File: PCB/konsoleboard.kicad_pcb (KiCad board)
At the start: 2 copper layers, 73.8 x 116.7 mm, 12 parts, among them SW1 SW_Wuerth_450301014042, SW10 SW_Push, SW2 SW_Push, SW3 SW_Wuerth_450301014042, SW5 SW_Push, SW6 SW_Push, SW7 SW_Push, SW8 SW_Push, SW9 SW_Wuerth_450301014042, U3 CR2013-MI2120

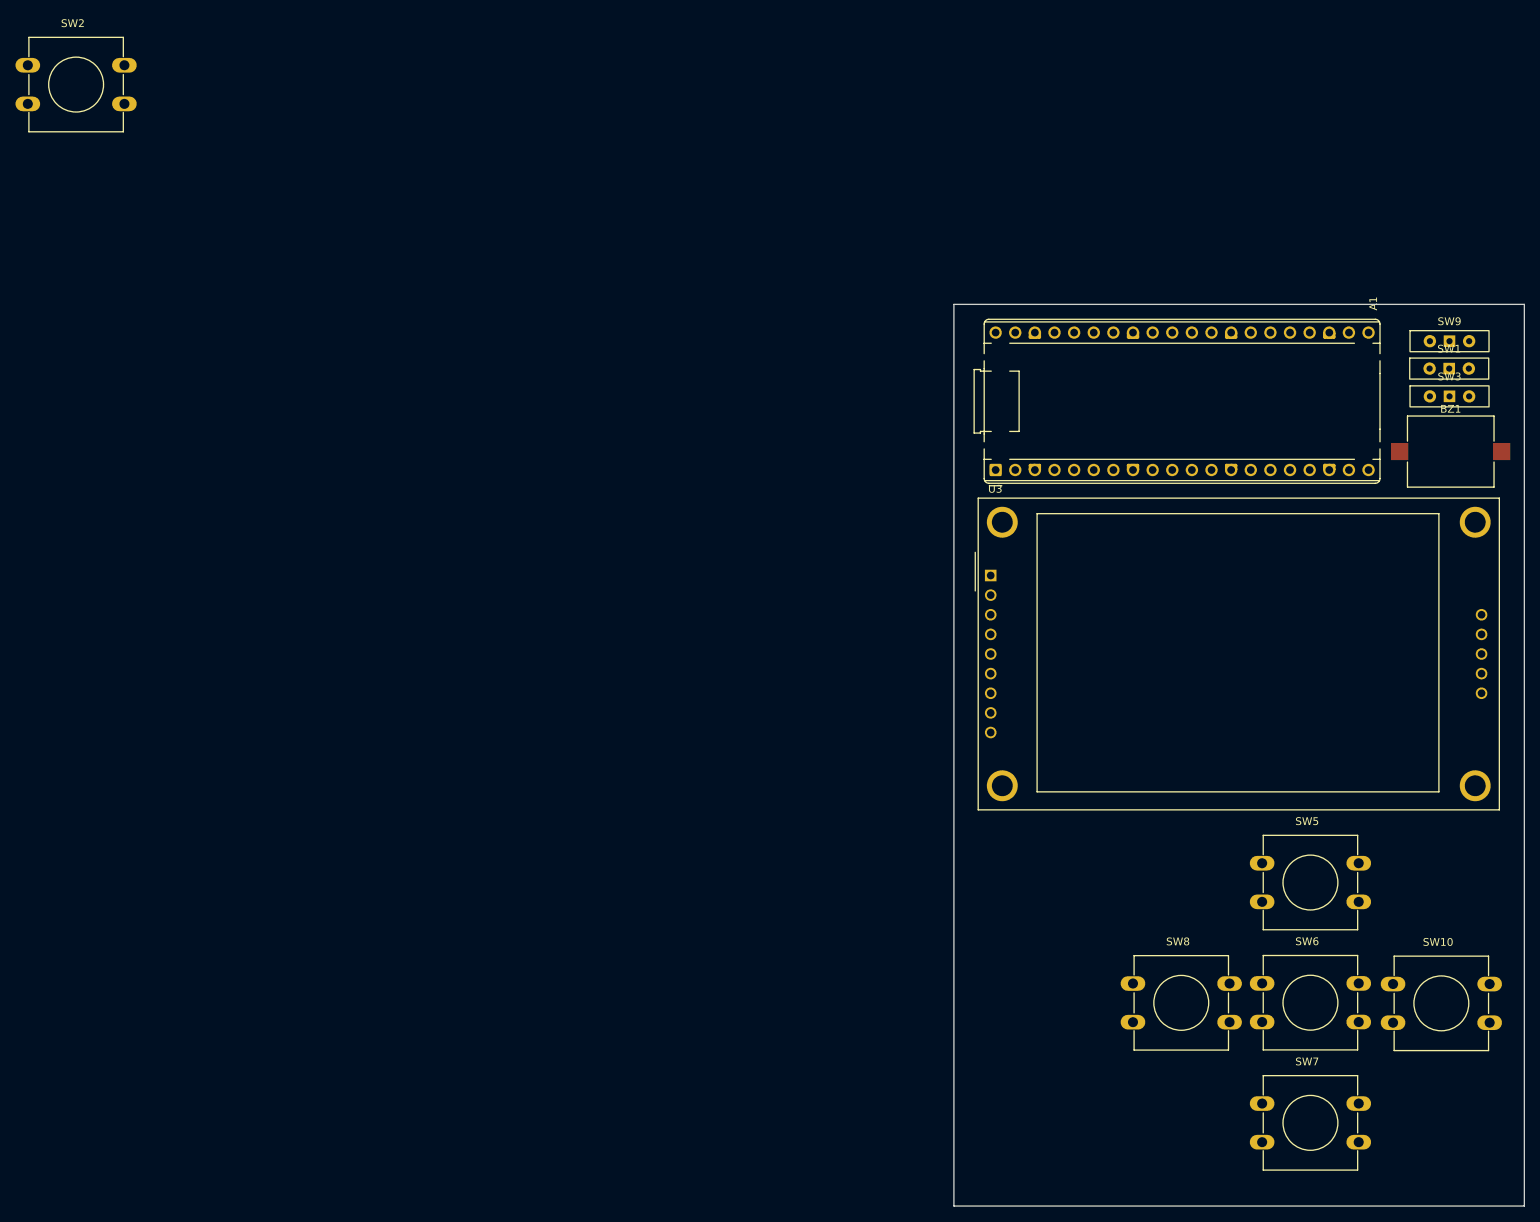
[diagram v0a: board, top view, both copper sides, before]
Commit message: Completed the pcb routing
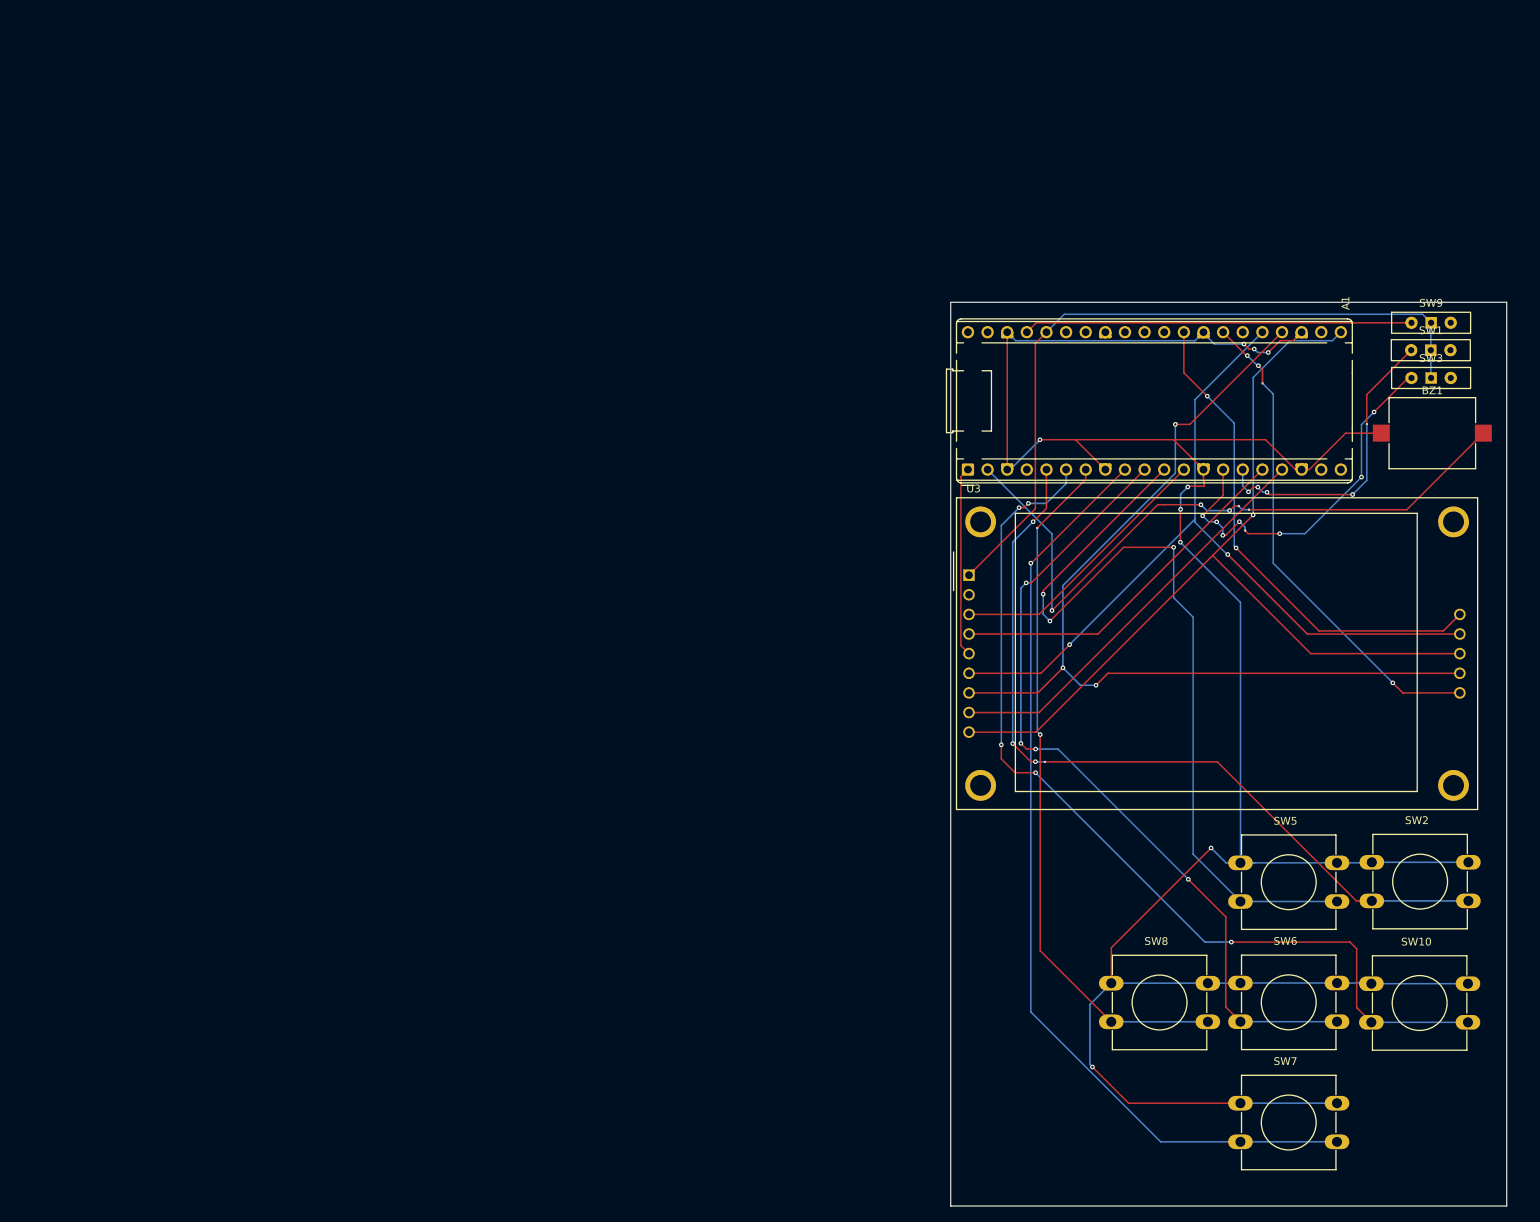
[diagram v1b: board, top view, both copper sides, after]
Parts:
- moved SW2 202.2 mm to (175.5, 107.9)
- moved A1 3.58 mm to (123.3, 57.1)
- moved SW3 3.37 mm to (183.2, 45.2)
- moved SW9 3.37 mm to (183.2, 38.1)
- moved BZ1 3.37 mm to (183.4, 52.4)
- moved SW1 3.37 mm to (183.2, 41.6)
- moved SW5 2.81 mm to (158.5, 108.0)
- moved SW6 2.81 mm to (158.5, 123.5)
- moved SW7 2.81 mm to (158.5, 139.1)
- moved U3 2.81 mm to (123.4, 70.8)
- moved SW10 2.81 mm to (175.5, 123.6)
- moved SW8 2.81 mm to (141.8, 123.6)
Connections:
- A1 pad 1: SDA2 -> Net-(A1-GPIO0)
- A1 pad 10: RP3 -> RP2
- A1 pad 11: RP4 -> RP1
- A1 pad 12: RP5 -> Net-(A1-GPIO9)
- A1 pad 14: SDA -> GameToggleSwitch
- A1 pad 15: SCL -> BuzzerToggleSwitch
- A1 pad 16: BuzzerP -> Net-(A1-GPIO12)
- A1 pad 17: unconnected-(A1-GPIO13-Pad17) -> Net-(A1-GPIO13)
- A1 pad 2: SCL2 -> BuzzerP
- A1 pad 21: BuzzerToggleSwitch -> MISO
- A1 pad 22: GameToggleSwitch -> unconnected-(A1-GPIO17-Pad22)
- A1 pad 24: unconnected-(A1-GPIO18-Pad24) -> SCK
- A1 pad 25: unconnected-(A1-GPIO19-Pad25) -> MOSI
- A1 pad 27: unconnected-(A1-GPIO21-Pad27) -> FLASH_CD
- A1 pad 29: unconnected-(A1-GPIO22-Pad29) -> SD_CS
- A1 pad 37: ToggleSwitch -> PowerToggleSwitch
- A1 pad 5: unconnected-(A1-GPIO3-Pad5) -> RP6
- A1 pad 6: RP6 -> RP5
- A1 pad 7: RP1 -> RP4
- A1 pad 9: RP2 -> RP3
- U3 pad 1: unconnected-(U3-VCC-Pad1) -> +3V3
- U3 pad 10: unconnected-(U3-SD_CS-Pad10) -> SD_CS
- U3 pad 11: unconnected-(U3-SD_MOSI-Pad11) -> MOSI
- U3 pad 12: unconnected-(U3-SD_MISO-Pad12) -> MISO
- U3 pad 13: unconnected-(U3-SD_SCK-Pad13) -> SCK
- U3 pad 14: unconnected-(U3-FLASH_CD-Pad14) -> FLASH_CD
- U3 pad 3: unconnected-(U3-~{CS}-Pad3) -> Net-(A1-GPIO9)
- U3 pad 4: unconnected-(U3-RESET-Pad4) -> Net-(A1-GPIO12)
- U3 pad 5: unconnected-(U3-D/~{C}-Pad5) -> Net-(A1-GPIO0)
- U3 pad 6: unconnected-(U3-MOSI-Pad6) -> MOSI
- U3 pad 7: unconnected-(U3-SCK-Pad7) -> SCK
- U3 pad 8: unconnected-(U3-LED-Pad8) -> Net-(A1-GPIO13)
- U3 pad 9: unconnected-(U3-MISO-Pad9) -> MISO
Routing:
- net GND: track 0.00 -> 330.9 mm, vias 0 -> 9
- net SCK: track 0.00 -> 123.0 mm, vias 0 -> 3
- net RP3: track 0.00 -> 121.9 mm, vias 0 -> 1
- net RP5: track 0.00 -> 121.6 mm, vias 0 -> 5
- net MISO: track 0.00 -> 117.2 mm, vias 0 -> 1
- net RP1: track 0.00 -> 108.3 mm, vias 0 -> 3
- net MOSI: track 0.00 -> 106.0 mm, vias 0 -> 2
- net RP2: track 0.00 -> 105.1 mm, vias 0 -> 4
- net RP6: track 0.00 -> 104.7 mm, vias 0 -> 4
- net +3V3: track 0.00 -> 94.0 mm
- net RP4: track 0.00 -> 90.5 mm, vias 0 -> 2
- net BuzzerP: track 0.00 -> 88.0 mm, vias 0 -> 5
- net SD_CS: track 0.00 -> 65.0 mm, vias 0 -> 2
- net FLASH_CD: track 0.00 -> 63.8 mm, vias 0 -> 4
- net Net-(A1-GPIO13): track 0.00 -> 53.5 mm
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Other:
- board size 73.8 x 116.7 mm -> 71.9 x 117 mm
